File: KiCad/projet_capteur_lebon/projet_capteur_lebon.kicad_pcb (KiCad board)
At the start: 2 copper layers, 68.6 x 53.3 mm, 9 parts, among them J1 Power, J2 Digital/PWM, J3 Analog, J4 Digital/PWM

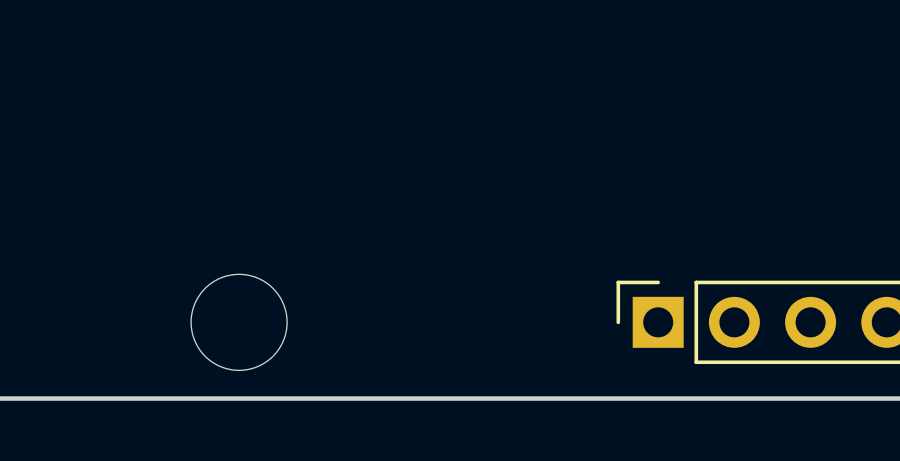
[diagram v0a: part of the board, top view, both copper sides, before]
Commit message: mep modele 3d flex s
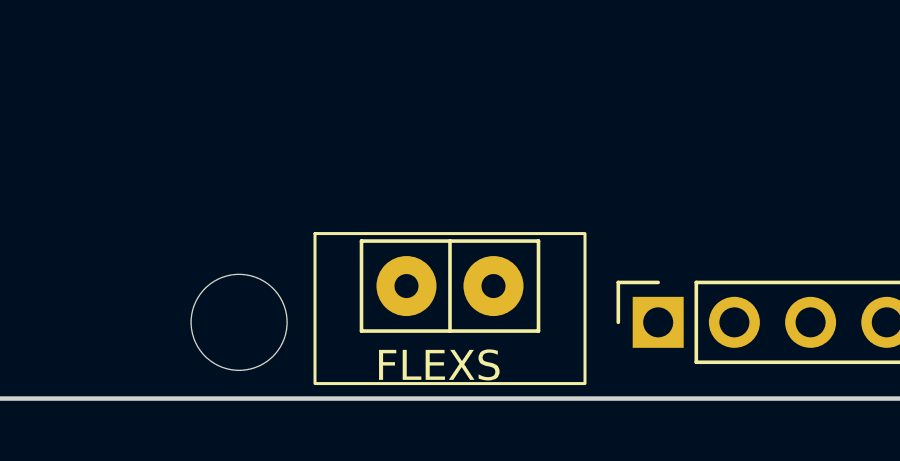
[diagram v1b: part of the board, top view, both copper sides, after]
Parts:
- added U2: ~, librairie_empreintes:SIP-2, F.Cu at (121.0, 97.0)
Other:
- board text removed: "ICSP"
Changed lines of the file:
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@@
 	(net 31 "unconnected-(U1-GND-Pad1)")
 	(net 32 "unconnected-(U1-VCC-Pad2)")
+	(net 33 "unconnected-(U2-VCC-Pad2)")
+	(net 34 "unconnected-(U2-GND-Pad1)")
 	(footprint "Connector_PinSocket_2.54mm:PinSocket_1x08_P2.54mm_Vertical"
 		(locked yes)
@@
 		(embedded_fonts no)
 	)
+	(footprint "librairie_empreintes:SIP-2"
+		(layer "F.Cu")
+		(at 121 97)
+		(property "Reference" "U2"
+			(at 0 1.75 0)
+			(layer "F.SilkS")
+			(hide yes)
+			(effects
+				(font
+					(size 1 1)
+					(thickness 0.15)
+				)
+			)
+		)
+		(property "Value" "~"
+			(at 0 -3.25 0)
+			(layer "F.Fab")
+			(hide yes)
+			(effects
+				(font
+					(size 1 1)
+					(thickness 0.15)
+				)
+			)
+		)
+		(property "Datasheet" ""
+			(at 0 -0.75 0)
+			(layer "F.Fab")
+			(hide yes)
+			(effects
+				(font
+					(size 1.27 1.27)
+					(thickness 0.15)
+				)
+			)
+		)
+		(property "Description" ""
+			(at 0 -0.75 0)
+			(layer "F.Fab")
+			(hide yes)
+			(effects
+				(font
+					(size 1.27 1.27)
+					(thickness 0.15)
+				)
+			)
+		)
+		(sheetname "/")
+		(sheetfile "projet_capteur_lebon.kicad_sch")
+		(attr through_hole)
+		(fp_line
+			(start -2.95 -2.25)
+			(end 2.95 -2.25)
+			(stroke
+				(width 0.12)
+				(type default)
+			)
+			(layer "F.SilkS")
+		)
+		(fp_line
+			(start -2.95 0.75)
+			(end -2.95 -2.25)
+			(stroke
+				(width 0.12)
+				(type default)
+			)
+			(layer "F.SilkS")
+		)
+		(fp_line
+			(start 0 -2.25)
+			(end 0 0.75)
+			(stroke
+				(width 0.12)
+				(type default)
+			)
+			(layer "F.SilkS")
+		)
+		(fp_line
+			(start 2.95 -2.25)
+			(end 2.95 0.75)
+			(stroke
+				(width 0.12)
+				(type default)
+			)
+			(layer "F.SilkS")
+		)
+		(fp_line
+			(start 2.95 0.75)
+			(end -2.95 0.75)
+			(stroke
+				(width 0.12)
+				(type default)
+			)
+			(layer "F.SilkS")
+		)
+		(fp_rect
+			(start -4.5 -2.5)
+			(end 4.5 2.5)
+			(stroke
+				(width 0.1)
+				(type default)
+			)
+			(fill no)
+			(layer "F.SilkS")
+		)
+		(fp_line
+			(start -2.7 -2)
+			(end 2.7 -2)
+			(stroke
+				(width 0.05)
+				(type default)
+			)
+			(layer "F.CrtYd")
+		)
+		(fp_line
+			(start -2.7 0.5)
+			(end -2.7 -2)
+			(stroke
+				(width 0.05)
+				(type default)
+			)
+			(layer "F.CrtYd")
+		)
+		(fp_line
+			(start 2.7 -2)
+			(end 2.7 0.5)
+			(stroke
+				(width 0.05)
+				(type default)
+			)
+			(layer "F.CrtYd")
+		)
+		(fp_line
+			(start 2.7 0.5)
+			(end -2.7 0.5)
+			(stroke
+				(width 0.05)
+				(type default)
+			)
+			(layer "F.CrtYd")
+		)
+		(fp_text user "FLEXS"
+			(at -2.5 2.5 0)
+			(unlocked yes)
+			(layer "F.SilkS")
+			(effects
+				(font
+					(size 1 1)
+					(thickness 0.1)
+				)
+				(justify left bottom)
+			)
+		)
+		(pad "1" thru_hole circle
+			(at -1.45 -0.75)
+			(size 2 2)
+			(drill 0.8)
+			(layers "*.Cu" "*.Mask")
+			(remove_unused_layers no)
+			(net 34 "unconnected-(U2-GND-Pad1)")
+			(pinfunction "GND")
+			(pintype "input")
+		)
+		(pad "2" thru_hole circle
+			(at 1.45 -0.75)
+			(size 2 2)
+			(drill 0.8)
+			(layers "*.Cu" "*.Mask")
+			(remove_unused_layers no)
+			(net 33 "unconnected-(U2-VCC-Pad2)")
+			(pinfunction "VCC")
+			(pintype "input")
+		)
+		(embedded_fonts no)
+		(model "C:/Users/clara/OneDrive/Documents/INSA/4A/Capteurs/2024-2025-4GP-Anatolie-Clara/KiCad/Modele 3D/FS-L-0095-103-ST - Assembly.stp"
+			(offset
+				(xyz 0 1.5 0)
+			)
+			(scale
+				(xyz 1 1 1)
+			)
+			(rotate
+				(xyz -0 -0 -0)
+			)
+		)
+	)
 	(footprint "Arduino_MountingHole:MountingHole_3.2mm"
 		(locked yes)
@@
 		(layer "Dwgs.User")
 	)
-	(gr_rect
-		(start 162.357 68.25)
-		(end 167.437 75.87)
-		(stroke
-			(width 0.15)
-			(type solid)
-		)
-		(fill no)
-		(layer "Dwgs.User")
-	)
 	(gr_line
 		(start 98.095 87.935)
@@
 		(layer "Edge.Cuts")
 	)
-	(gr_text "ICSP"
-		(at 164.897 72.06 90)
-		(layer "Dwgs.User")
-		(effects
-			(font
-				(size 1 1)
-				(thickness 0.15)
-			)
-		)
-	)
 	(embedded_fonts no)
